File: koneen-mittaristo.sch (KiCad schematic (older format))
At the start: 21 parts, among them J1 30A, J2 J1, J4 J2

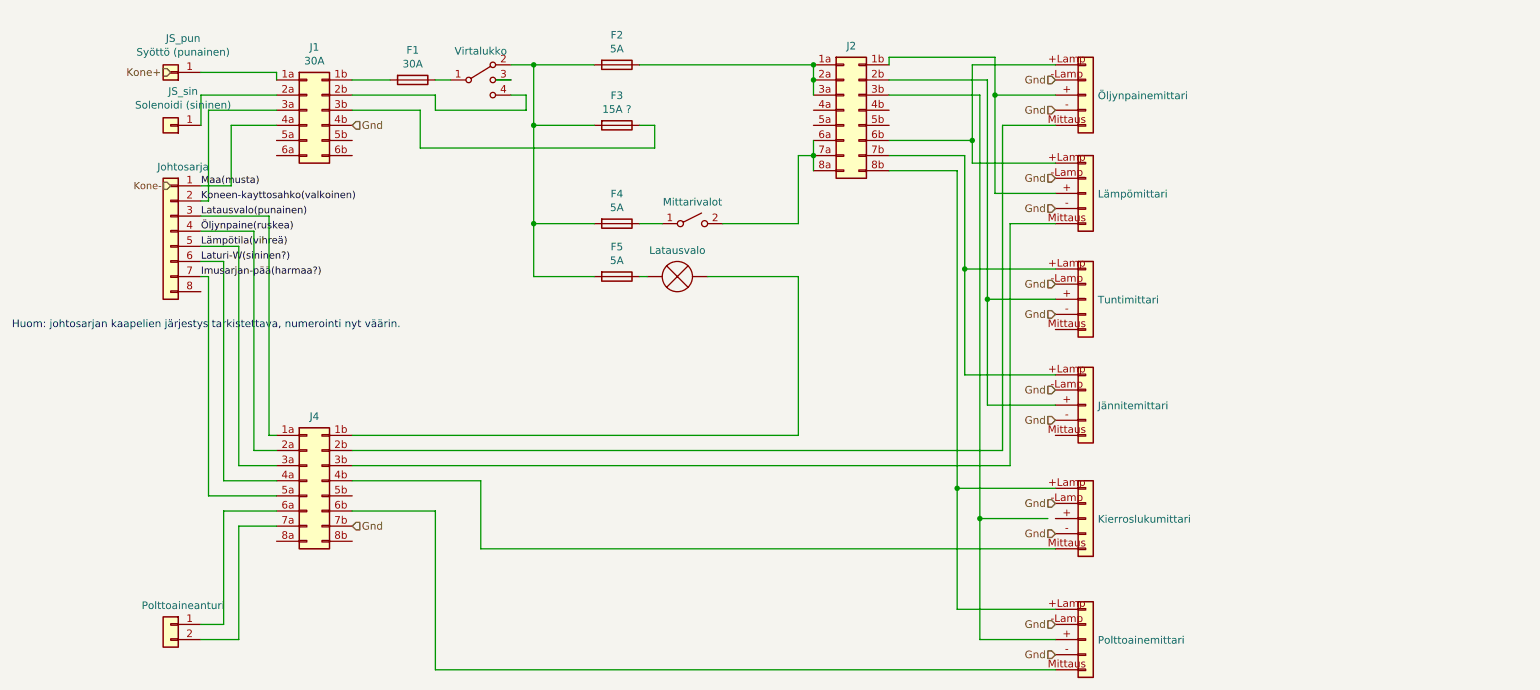
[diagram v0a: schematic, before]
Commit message: Koneen sähköpiirros järjestetty uudelleen
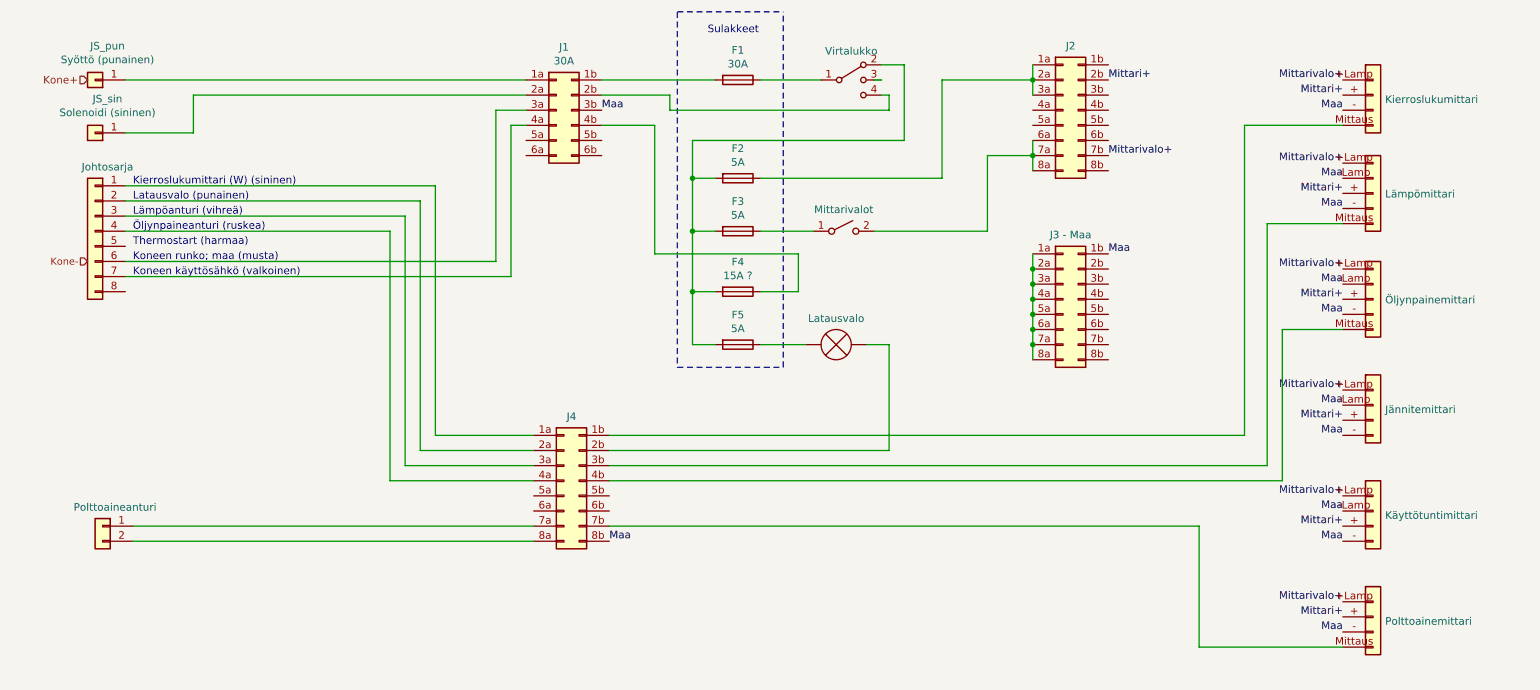
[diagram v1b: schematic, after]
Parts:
- removed Jännitemittari, Kierroslukumittari, Lämpömittari, Polttoainemittari, Tuntimittari, Öljynpainemittari: Koneen-mittari-1-mittausnapa, symbol SL-sahkot-rescue:Koneen-mittari-1-mittausnapa-Connector_Generic
- added J3: J3 - Maa, symbol Connector_Generic:Conn_02x08_Row_Letter_Last
- added Jännitemittari, Käyttötuntimittari: Koneen-mittari-4-nap-ei-mittausta, symbol SL-sahkot-rescue:Koneen-mittari-4-nap-ei-mittausta
- added Kierroslukumittari, Polttoainemittari: Koneen-mittari-4-nap, symbol SL-sahkot-rescue:Koneen-mittari-4-nap
- added Lämpömittari, Öljynpainemittari: Koneen-mittari-5-nap, symbol SL-sahkot-rescue:Koneen-mittari-5-nap
- F3: value 15A ? -> 5A
- F4: value 5A -> 15A ?
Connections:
- net Mittari+: now reaches J2.2b (Pin_2b)
- net Mittari+: now also Jännitemittari.+ (Pin_3), Kierroslukumittari.+ (Pin_3), Käyttötuntimittari.+ (Pin_3), Lämpömittari.+ (Pin_3), Polttoainemittari.+ (Pin_3), Öljynpainemittari.+ (Pin_3)
- net Mittarivalo+: now reaches J2.7b (Pin_7b)
- net Mittarivalo+: now also Jännitemittari.+Lamp (Pin_1), Kierroslukumittari.+Lamp (Pin_1), Käyttötuntimittari.+Lamp (Pin_1), Lämpömittari.+Lamp (Pin_1), Polttoainemittari.+Lamp (Pin_1), Öljynpainemittari.+Lamp (Pin_1)
- net at J4.2b (Pin_2b): now also Latausvalo.2 (+)
- net at J4.1b (Pin_1b): now also Kierroslukumittari.Mittaus (Pin_5); no longer Latausvalo.2 (+)
- net at J4.3b (Pin_3b): now also Lämpömittari.Mittaus (Pin_5)
- net at J4.4b (Pin_4b): now also Öljynpainemittari.Mittaus (Pin_5)
- net at J4.6a (Pin_6a): no longer Polttoaineanturi.1 (Pin_1)
- net at J4.7a (Pin_7a): now also Polttoaineanturi.1 (Pin_1); no longer Polttoaineanturi.2 (Pin_2)
- net at J4.8a (Pin_8a): now also Polttoaineanturi.2 (Pin_2)
- net Maa: now reaches J4.8b (Pin_8b)
- net Maa: now also J1.3b (Pin_3b), J3.1b (Pin_1b), Jännitemittari.- (Pin_4), Jännitemittari.-Lamp (Pin_5), Kierroslukumittari.- (Pin_4), Käyttötuntimittari.- (Pin_4), Käyttötuntimittari.-Lamp (Pin_5), Lämpömittari.- (Pin_4), Lämpömittari.-Lamp (Pin_2), Polttoainemittari.- (Pin_4), Öljynpainemittari.- (Pin_4), Öljynpainemittari.-Lamp (Pin_2)
- net at Mittarivalot.1 (A): now also F3.1; no longer F4.1
- net Gnd: no longer names the net of J4.7b (Pin_7b)
- net Gnd: now also Polttoainemittari.Mittaus (Pin_5); no longer J1.4b (Pin_4b)
- net Imusarjan-pää(harmaa?): no longer names the net of J4.5a (Pin_5a)
- net Imusarjan-pää(harmaa?): no longer Johtosarja.7 (Pin_7)
- net Koneen-kayttosahko(valkoinen): no longer names the net of Johtosarja.2 (Pin_2)
- net Koneen-kayttosahko(valkoinen): now also J4.2a (Pin_2a); no longer J1.3a (Pin_3a)
- net Latausvalo(punainen): no longer names the net of J4.1a (Pin_1a)
- net Latausvalo(punainen): now also Johtosarja.1 (Pin_1); no longer Johtosarja.3 (Pin_3)
- net Laturi-W(sininen?): no longer names the net of J4.4a (Pin_4a)
- net Laturi-W(sininen?): now also Johtosarja.4 (Pin_4); no longer Johtosarja.6 (Pin_6)
- net Lämpötila(vihreä): no longer names the net of J4.3a (Pin_3a)
- net Lämpötila(vihreä): now also Johtosarja.3 (Pin_3); no longer Johtosarja.5 (Pin_5)
- net Maa(musta): no longer names the net of J1.4a (Pin_4a)
- net Maa(musta): now also Johtosarja.7 (Pin_7); no longer Johtosarja.1 (Pin_1)
- removed net Öljynpaine(ruskea): J4.2a (Pin_2a), Johtosarja.4 (Pin_4)
- new net: J1.3a (Pin_3a), Johtosarja.6 (Pin_6)
- new net: F4.1, J1.4b (Pin_4b)
- new net: J3.1a (Pin_1a), J3.2a (Pin_2a), J3.3a (Pin_3a), J3.4a (Pin_4a), J3.5a (Pin_5a), J3.6a (Pin_6a), J3.7a (Pin_7a), J3.8a (Pin_8a)
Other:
- note added: "Kierroslukumittari (W) (sininen)"
- note added: "Koneen käyttösähkö (valkoinen)"
- note added: "Koneen runko; maa (musta)"
- note added: "Latausvalo (punainen)"
- note added: "Lämpöanturi (vihreä)"
- note added: "Sulakkeet"
- note added: "Thermostart (harmaa)"
- note added: "Öljynpaineanturi (ruskea)"
- note removed: "Huom: johtosarjan kaapelien järjestys tarkistettava, numerointi nyt väärin."
- moved on the sheet: F1, F2, F3, F4, F5, J1, J2, J4, JS_pun, JS_sin, Johtosarja, Latausvalo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
